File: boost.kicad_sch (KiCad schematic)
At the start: 9 parts

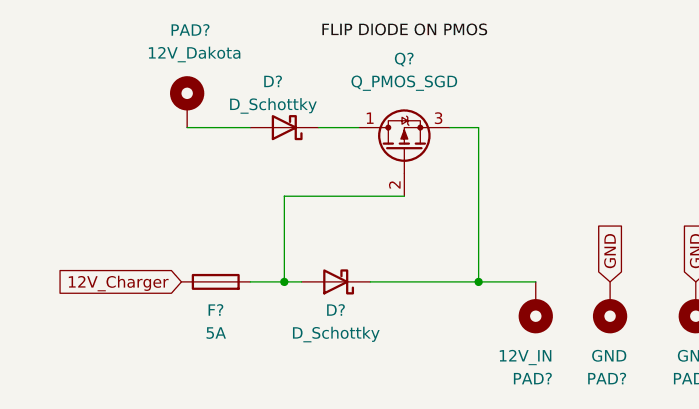
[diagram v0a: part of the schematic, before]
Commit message: Finished Schematic?
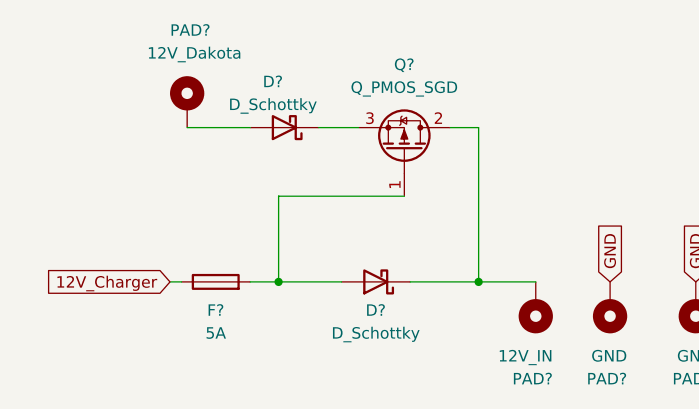
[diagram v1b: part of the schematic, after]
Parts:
- Q?: footprint SamacSys_Parts:BTS3035TFATMA1 -> (none); symbol Device:Q_PMOS_DGS -> Device:Q_PMOS_GDS
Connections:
- net at Q?.1 (G): now also D?.2 (A), F?.2; no longer D?.1 (K)
- net at D?.1 (K), PAD?.1: now also Q?.2 (D); no longer Q?.3 (S)
- new net: D?.1 (K), Q?.3 (S)
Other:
- moved on the sheet: D?, Q?
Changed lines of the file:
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@@
   (junction (at 139.7 85.09) (diameter 0) (color 0 0 0 0)
   )
-  (junction (at 118.11 85.09) (diameter 0) (color 0 0 0 0)
+  (junction (at 117.475 85.09) (diameter 0) (color 0 0 0 0)
+  )
+  (wire (pts (xy 105.41 85.09) (xy 106.68 85.09))
+    (stroke (width 0) (type default) (color 0 0 0 0))
   )
   (wire (pts (xy 139.7 85.09) (xy 146.05 85.09))
@@
     (stroke (width 0) (type default) (color 0 0 0 0))
   )
-  (wire (pts (xy 114.3 85.09) (xy 118.11 85.09))
+  (wire (pts (xy 114.3 85.09) (xy 117.475 85.09))
+    (stroke (width 0) (type default) (color 0 0 0 0))
+  )
+  (wire (pts (xy 117.475 75.565) (xy 117.475 85.09))
     (stroke (width 0) (type default) (color 0 0 0 0))
   )
@@
     (stroke (width 0) (type default) (color 0 0 0 0))
   )
-  (wire (pts (xy 118.11 75.565) (xy 118.11 85.09))
+  (wire (pts (xy 131.445 75.565) (xy 117.475 75.565))
     (stroke (width 0) (type default) (color 0 0 0 0))
   )
@@
     (stroke (width 0) (type default) (color 0 0 0 0))
   )
-  (wire (pts (xy 118.11 85.09) (xy 120.015 85.09))
-    (stroke (width 0) (type default) (color 0 0 0 0))
-  )
-  (wire (pts (xy 131.445 75.565) (xy 118.11 75.565))
+  (wire (pts (xy 117.475 85.09) (xy 124.46 85.09))
     (stroke (width 0) (type default) (color 0 0 0 0))
   )
@@
     (stroke (width 0) (type default) (color 0 0 0 0))
   )
-  (wire (pts (xy 127.635 85.09) (xy 139.7 85.09))
+  (wire (pts (xy 132.08 85.09) (xy 139.7 85.09))
     (stroke (width 0) (type default) (color 0 0 0 0))
-  )
-  (label "FLIP DIODE ON PMOS" (at 122.174 58.166 0)
-    (effects (font (size 1.27 1.27)) (justify left bottom))
   )
   (global_label "GND" (shape input) (at 163.83 85.09 90) (fields_autoplaced)
@@
     )
   )
-  (global_label "12V_Charger" (shape input) (at 106.68 85.09 180) (fields_autoplaced)
+  (global_label "12V_Charger" (shape input) (at 105.41 85.09 180) (fields_autoplaced)
     (effects (font (size 1.27 1.27)) (justify right))
-    (property "Intersheet References" "${INTERSHEET_REFS}" (id 0) (at 92.4136 85.0106 0)
+    (property "Intersheet References" "${INTERSHEET_REFS}" (id 0) (at 91.1436 85.0106 0)
       (effects (font (size 1.27 1.27)) (justify right) hide)
     )
@@
     (pin "1")
   )
-  (symbol (lib_id "Device:Q_PMOS_DGS") (at 131.445 70.485 90) (unit 1)
+  (symbol (lib_id "Device:Q_PMOS_GDS") (at 131.445 70.485 270) (mirror x) (unit 1)
     (in_bom yes) (on_board yes) (fields_autoplaced)
-    (property "Reference" "Q?" (id 0) (at 131.445 60.325 90))
-    (property "Value" "Q_PMOS_SGD" (id 1) (at 131.445 62.865 90))
-    (property "Footprint" "SamacSys_Parts:BTS3035TFATMA1" (id 2) (at 128.905 65.405 0)
+    (property "Reference" "Q?" (id 0) (at 131.445 60.96 90))
+    (property "Value" "Q_PMOS_SGD" (id 1) (at 131.445 63.5 90))
+    (property "Footprint" "" (id 2) (at 133.985 65.405 0)
       (effects (font (size 1.27 1.27)) hide)
     )
-    (property "Datasheet" "~" (id 3) (at 131.445 70.485 0)
+    (property "Datasheet" "https://www.mouser.com/ProductDetail/Infineon-Technologies/IPD650P06NMATMA1?qs=unwgFEO1A6vz3T2Vr47kIg%3D%3D" (id 3) (at 131.445 70.485 0)
       (effects (font (size 1.27 1.27)) hide)
     )
@@
     (pin "1")
   )
-  (symbol (lib_id "Device:D_Schottky") (at 123.825 85.09 180) (unit 1)
+  (symbol (lib_id "Device:D_Schottky") (at 128.27 85.09 180) (unit 1)
     (in_bom yes) (on_board yes)
-    (property "Reference" "D?" (id 0) (at 123.825 88.265 0))
-    (property "Value" "D_Schottky" (id 1) (at 123.825 90.805 0))
-    (property "Footprint" "" (id 2) (at 123.825 85.09 0)
+    (property "Reference" "D?" (id 0) (at 128.27 88.265 0))
+    (property "Value" "D_Schottky" (id 1) (at 128.27 90.805 0))
+    (property "Footprint" "" (id 2) (at 128.27 85.09 0)
       (effects (font (size 1.27 1.27)) hide)
     )
-    (property "Datasheet" "~" (id 3) (at 123.825 85.09 0)
+    (property "Datasheet" "~" (id 3) (at 128.27 85.09 0)
       (effects (font (size 1.27 1.27)) hide)
     )

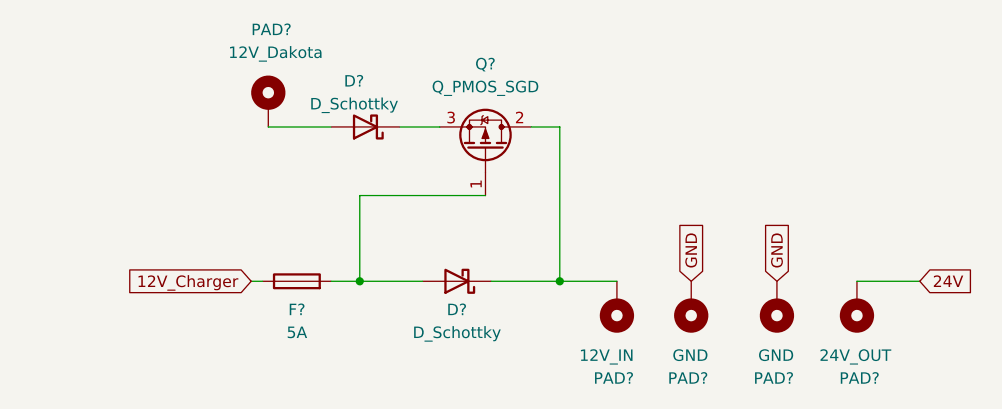
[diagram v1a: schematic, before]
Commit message: did basic layout
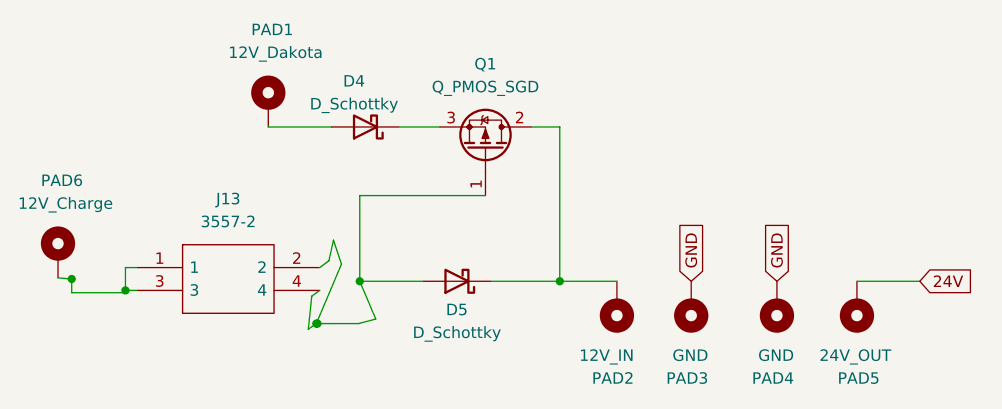
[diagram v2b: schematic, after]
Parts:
- removed F?: 5A, symbol Device:Fuse
- added J13: 3557-2, SamacSys_Parts:3557-2, symbol SamacSys_Parts:3557-2
- added PAD6: 12V_Charge, TestPoint:TestPoint_Pad_4.0x4.0mm, symbol Mechanical:MountingHole_Pad
- Q1: renamed from Q?; footprint (none) -> SamacSys_Parts:BTS3035TFATMA1
- gave numbers to parts that had none: 7
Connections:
- new net: J13.1, J13.3, PAD6.1
- new net: J13.2, J13.4

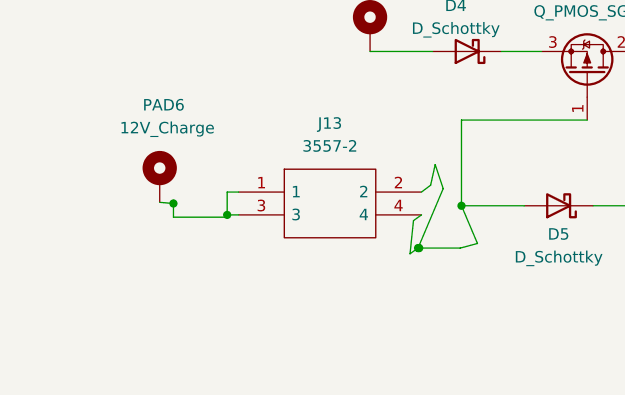
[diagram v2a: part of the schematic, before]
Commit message: more stuff done
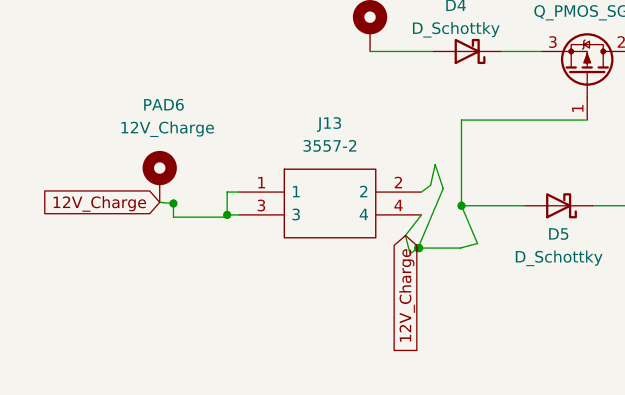
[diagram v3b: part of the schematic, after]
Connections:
- net 12V_Charge: now reaches J13.1, J13.3, PAD6.1
- net 12V_Charge: now also J13.2, J13.4
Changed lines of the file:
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@@
     (stroke (width 0) (type default) (color 0 0 0 0))
   )
-  (wire (pts (xy 111.76 90.424) (xy 112.141 86.741))
+  (wire (pts (xy 111.76 90.424) (xy 111.252 88.392))
     (stroke (width 0) (type default) (color 0 0 0 0))
   )
@@
     (stroke (width 0) (type default) (color 0 0 0 0))
   )
-  (wire (pts (xy 112.141 86.741) (xy 113.03 86.106))
+  (wire (pts (xy 111.252 88.392) (xy 113.03 86.106))
     (stroke (width 0) (type default) (color 0 0 0 0))
   )
@@
     )
   )
+  (global_label "12V_Charge" (shape input) (at 111.252 88.392 270) (fields_autoplaced)
+    (effects (font (size 1.27 1.27)) (justify right))
+    (property "Intersheet References" "${INTERSHEET_REFS}" (id 0) (at 111.3314 101.8722 90)
+      (effects (font (size 1.27 1.27)) (justify right) hide)
+    )
+  )
   (global_label "24V" (shape input) (at 179.705 85.09 0) (fields_autoplaced)
     (effects (font (size 1.27 1.27)) (justify left))
@@
     )
   )
+  (global_label "12V_Charge" (shape input) (at 83.947 84.709 180) (fields_autoplaced)
+    (effects (font (size 1.27 1.27)) (justify right))
+    (property "Intersheet References" "${INTERSHEET_REFS}" (id 0) (at 70.4668 84.7884 0)
+      (effects (font (size 1.27 1.27)) (justify right) hide)
+    )
+  )

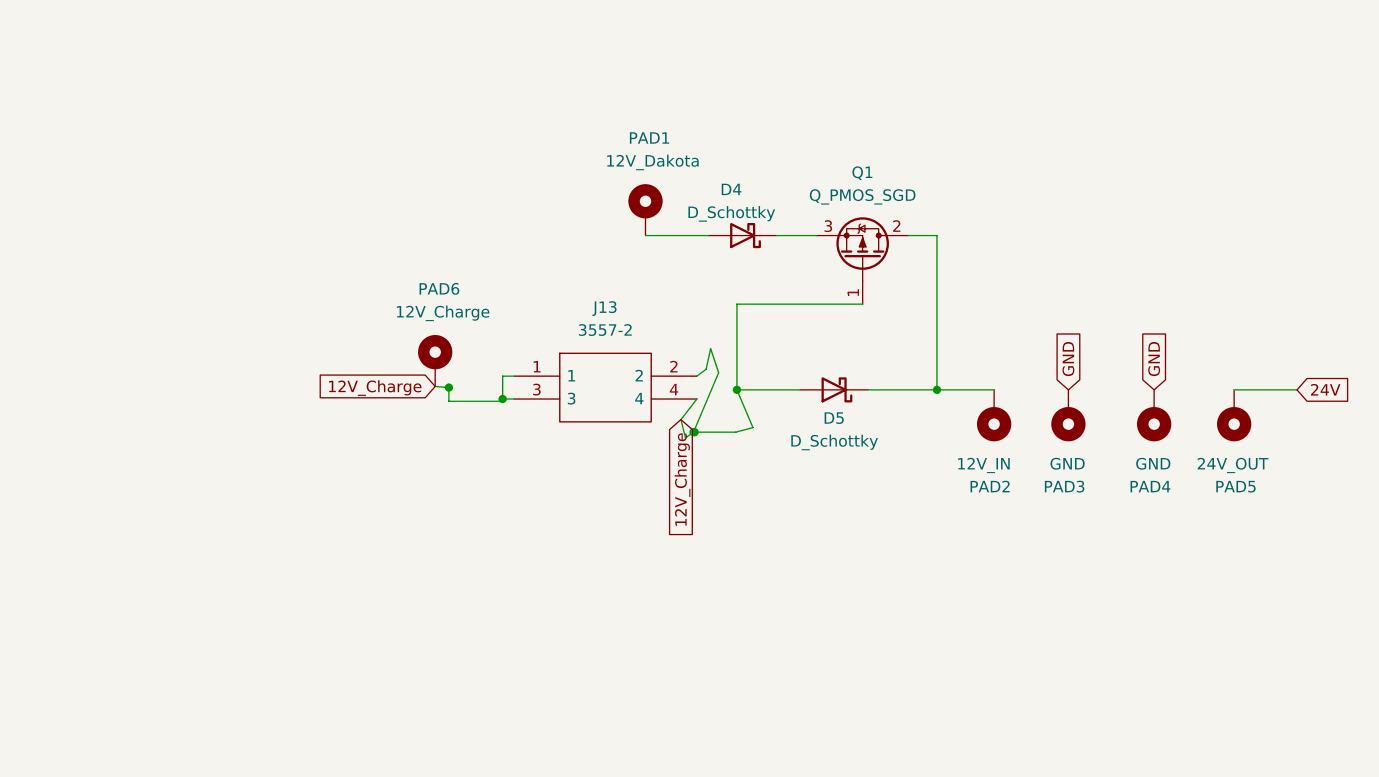
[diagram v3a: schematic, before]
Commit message: Done
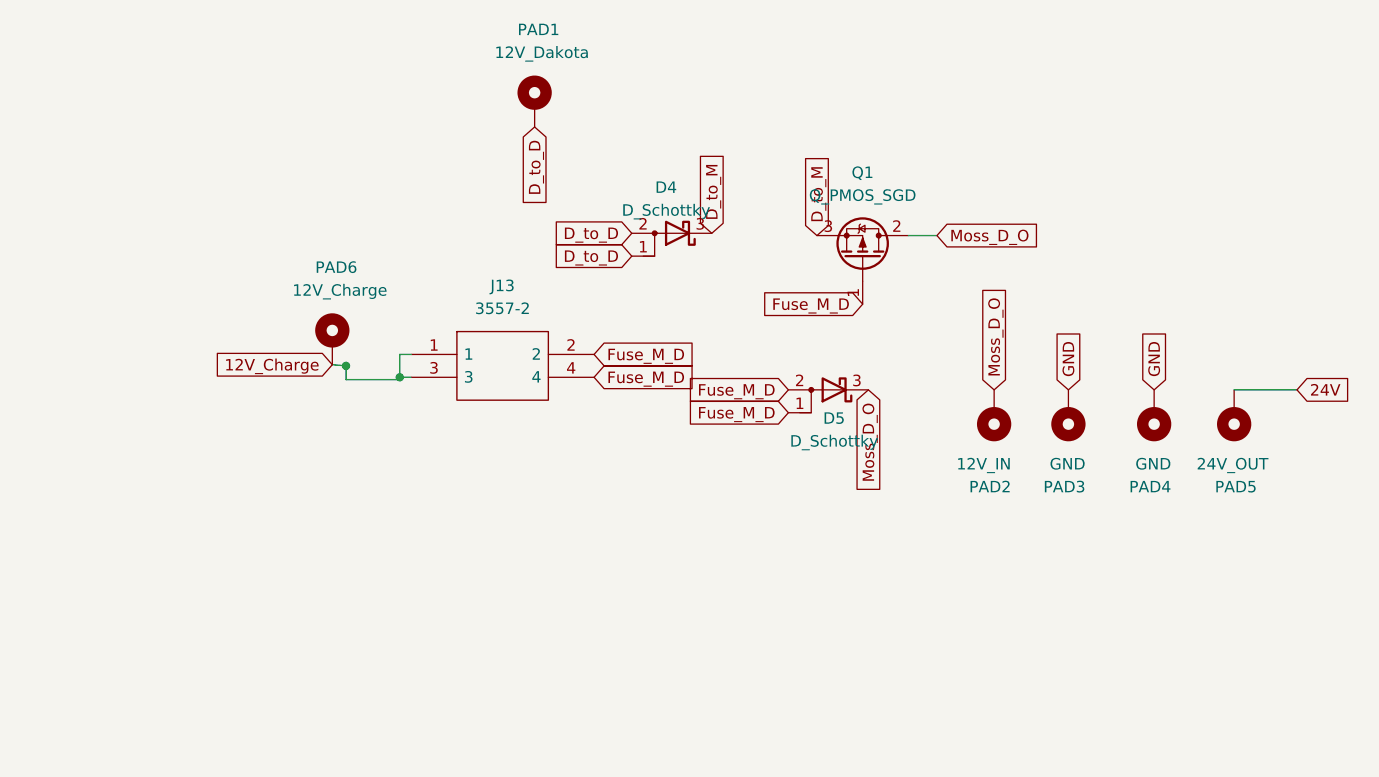
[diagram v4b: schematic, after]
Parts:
- D4, D5: footprint (none) -> SamacSys_Parts:RBQ10RSM10BTL1; symbol Device:D_Schottky -> Device:D_Schottky_AAK
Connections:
- net 12V_Charge: no longer J13.2, J13.4
- net D_to_D: now reaches D4.2 (A), PAD1.1
- net D_to_D: now also D4.1 (A)
- net Fuse_M_D: now reaches D5.2 (A), Q1.1 (G)
- net Fuse_M_D: now also D5.1 (A), J13.2, J13.4
- net Moss_D_O: now reaches PAD2.1, Q1.2 (D)
- net Moss_D_O: now also D5.3 (K); no longer D5.1 (K)
- net D_to_M: now reaches Q1.3 (S)
- net D_to_M: now also D4.3 (K); no longer D4.1 (K)
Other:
- moved on the sheet: J13, PAD1, PAD6

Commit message: Made corrections
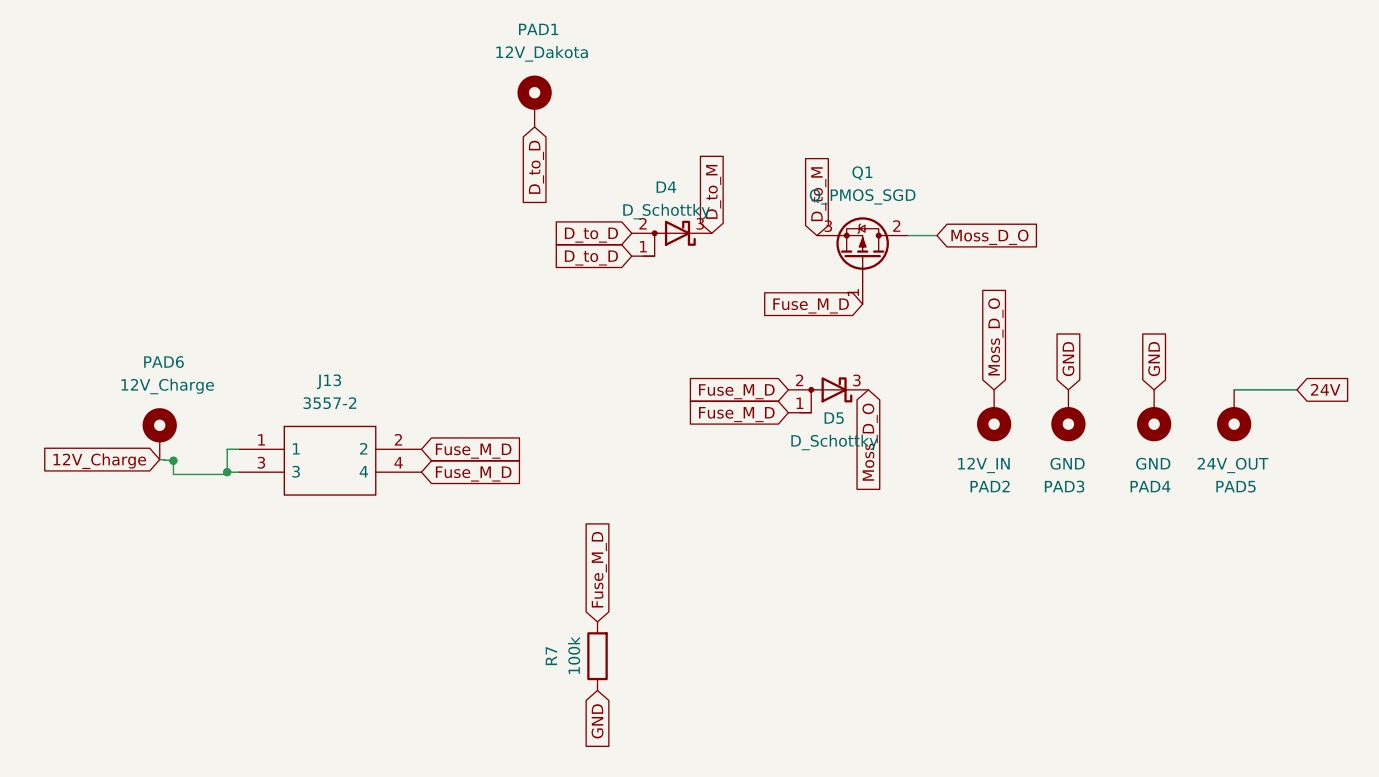
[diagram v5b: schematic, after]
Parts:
- added R7: 100k, Resistor_SMD:R_0603_1608Metric, symbol Device:R
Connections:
- net Fuse_M_D: now also R7.2
- net GND: now also R7.1
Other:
- moved on the sheet: J13, PAD6
